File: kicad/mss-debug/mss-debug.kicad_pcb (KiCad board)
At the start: 2 copper layers, 82.6 x 76.2 mm, 94 parts, among them J1 Screw_Terminal_01x02, J10 Screw_Terminal_01x02, J2 SM04B-SRSS, J3 SM04B-SRSS, J4 SM04B-SRSS, J5 8P8C, J6 8P8C, J7 AVR-ISP, J8 Screw_Terminal_01x02, J9 Screw_Terminal_01x02, U1 AP7381-50Y, U2 ATtiny861A-S, U3 74HC4049, U4 AP3012

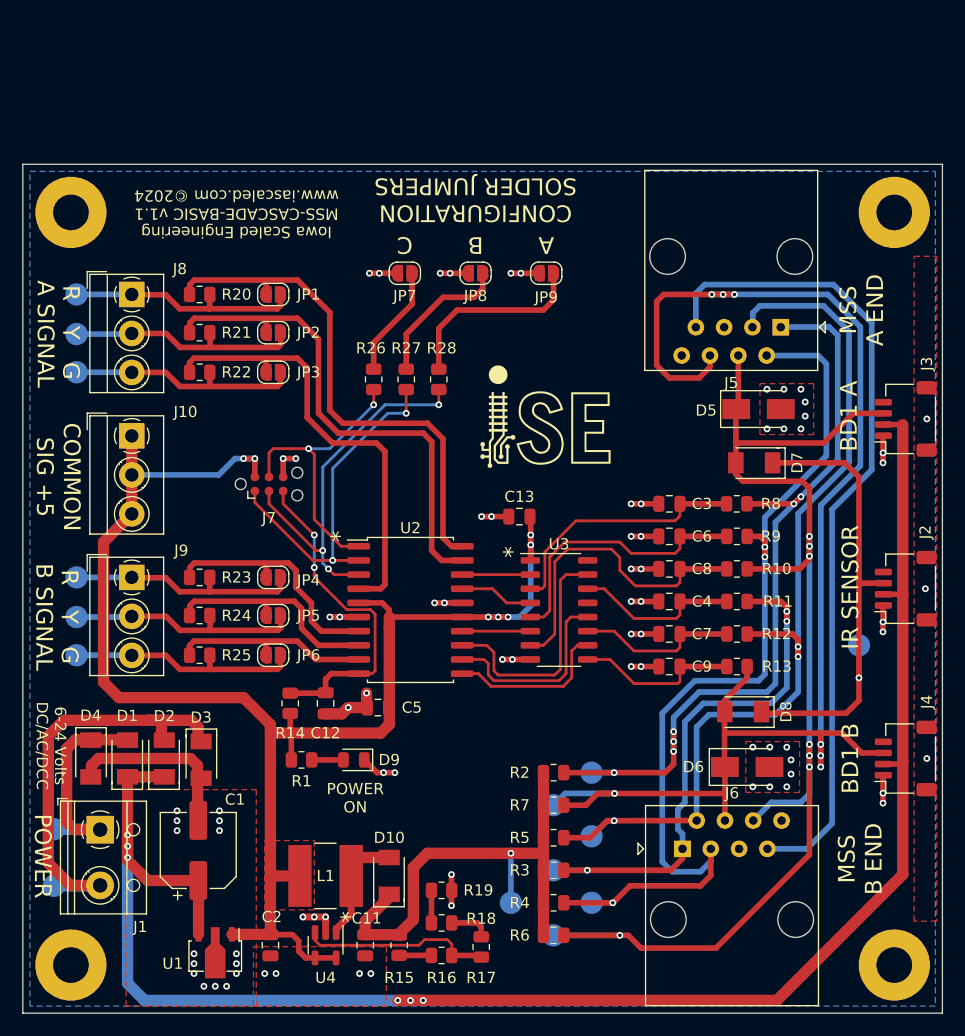
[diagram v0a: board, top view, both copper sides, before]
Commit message: Initial cut of the 2.0 board
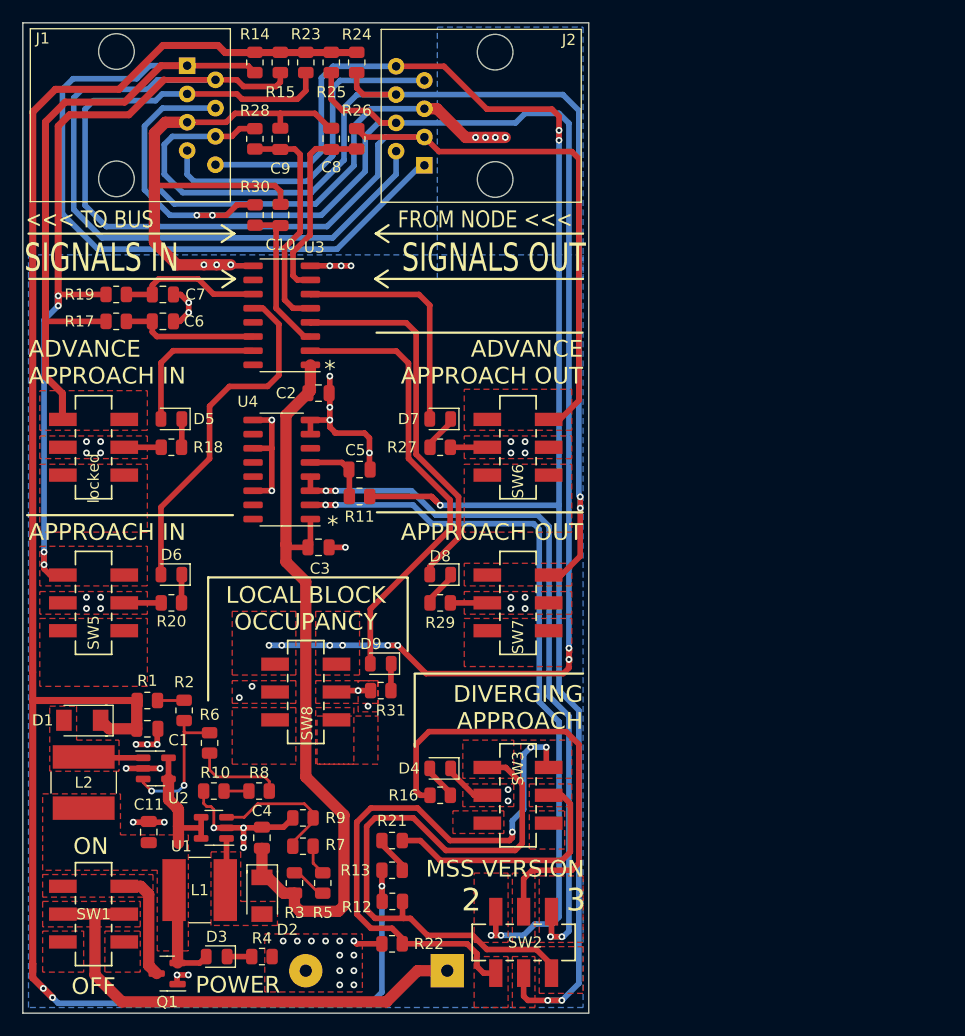
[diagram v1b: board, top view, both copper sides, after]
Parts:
- removed C12: 1uF, Capacitor_SMD:C_0805_2012Metric
- removed C13: 0.1uF, Capacitor_SMD:C_0805_2012Metric
- removed D10: CDBM140G, ISE_Generic:SOD-123T
- removed H1, H2, H3, H4: MountingHole, MountingHole:MountingHole_3.2mm_M3_Pad
- removed J10, J8, J9: Screw_Terminal_01x02, TerminalBlock_MetzConnect:TerminalBlock_MetzConnect_Type059_RT06303HBWC_1x03_P3.50mm_Horizontal
- removed J3, J4: SM04B-SRSS, Connector_JST:JST_SH_SM04B-SRSS-TB_1x04-1MP_P1.00mm_Horizontal
- removed J5, J6: 8P8C, Connector_RJ:RJ45_Amphenol_54602-x08_Horizontal
- removed J7: AVR-ISP, Connector:Tag-Connect_TC2030-IDC-NL_2x03_P1.27mm_Vertical
- removed JP1, JP2, JP3, JP4, JP5, JP6, JP7, JP8, JP9: SolderJumper_2_Open, Jumper:SolderJumper-2_P1.3mm_Open_RoundedPad1.0x1.5mm
- removed TP1, TP10, TP11, TP12, TP13, TP14, TP15, TP16, TP2, TP3, TP4, TP5, TP6, TP7, TP8, TP9: TestPoint, TestPoint:TestPoint_Pad_D2.0mm
- added BT1: Keystone 2479, Battery:BatteryHolder_Keystone_2479_3xAAA, B.Cu at (63.5, 188.0)
- added C10: 0.1uF, Capacitor_SMD:C_0805_2012Metric, F.Cu at (48.5, 120.1)
- added L2: 4.7uH, ISE_UltraLibrarian:MSS6132-xxxMLC, F.Cu at (30.9, 171.1)
- added Q1: Si2333, Package_TO_SOT_SMD:SOT-23, F.Cu at (38.4, 188.2)
- added R29: 1K, Resistor_SMD:R_0805_2012Metric, F.Cu at (62.9, 154.9)
- added R30: 10k, Resistor_SMD:R_0805_2012Metric, F.Cu at (46.2, 120.1)
- added R31: 1K, Resistor_SMD:R_0805_2012Metric, F.Cu at (57.5, 162.8)
- added SW1: JS202011SCQN, ISE_UltraLibrarian:SW_JS202011SCQN, F.Cu at (31.8, 182.9)
- added SW2: JS202011SCQN, ISE_UltraLibrarian:SW_JS202011SCQN, F.Cu at (70.4, 185.4)
- added SW3: JS202011SCQN, ISE_UltraLibrarian:SW_JS202011SCQN, F.Cu at (69.8, 172.2)
- added SW5: JS202011SCQN, ISE_UltraLibrarian:SW_JS202011SCQN, F.Cu at (31.8, 154.9)
- added SW6: JS202011SCQN, ISE_UltraLibrarian:SW_JS202011SCQN, F.Cu at (69.8, 141.0)
- added SW7: JS202011SCQN, ISE_UltraLibrarian:SW_JS202011SCQN, F.Cu at (69.8, 154.9)
- added SW8: JS202011SCQN, ISE_UltraLibrarian:SW_JS202011SCQN, F.Cu at (50.8, 162.9)
- added locked: JS202011SCQN, ISE_UltraLibrarian:SW_JS202011SCQN, F.Cu at (31.8, 141.0)
- C1: value 68uF -> 10uF; footprint Capacitor_SMD:CP_Elec_6.3x5.8 -> Capacitor_SMD:C_0805_2012Metric
- C11: value 10uF -> 22uF
- C2: value 22uF -> 0.1uF
- C4: value 0.1uF -> 10uF
- D3: value CDBM140G -> GREEN LED; footprint ISE_Generic:SOD-123T -> LED_SMD:LED_0805_2012Metric
- D4: value CDBM140G -> BLUE LED; footprint ISE_Generic:SOD-123T -> LED_SMD:LED_0805_2012Metric
- D5: value SMAJ18A-TP -> WHITE LED; footprint Diode_SMD:D_SMA -> LED_SMD:LED_0805_2012Metric
- D6: value SMAJ18A-TP -> YELLOW LED; footprint Diode_SMD:D_SMA -> LED_SMD:LED_0805_2012Metric
- D7: value CDBM140G -> WHITE LED; footprint ISE_Generic:SOD-123T -> LED_SMD:LED_0805_2012Metric
- D8: value CDBM140G -> YELLOW LED; footprint ISE_Generic:SOD-123T -> LED_SMD:LED_0805_2012Metric
- D9: value GREEN LED -> RED LED
- J1: value Screw_Terminal_01x02 -> 8P8C; footprint TerminalBlock_RND:TerminalBlock_RND_205-00012_1x02_P5.00mm_Horizontal -> Connector_RJ:RJ45_Amphenol_54602-x08_Horizontal
- J2: value SM04B-SRSS -> 8P8C; footprint Connector_JST:JST_SH_SM04B-SRSS-TB_1x04-1MP_P1.00mm_Horizontal -> Connector_RJ:RJ45_Amphenol_54602-x08_Horizontal
- R1, R17, R26, R28: value 1k -> 10k
- R10: value 10k -> 330
- R13, R16, R4, R6, R8: value 10k -> 1k
- R18, R27: value 1k -> 1K
- R19, R22, R23, R24, R25: value 330 -> 10k
- R20: value 330 -> 1K
- R21: value 330 -> 1k
- U1: value AP7381-50Y -> AP3012; footprint ISE_Generic:SOT-89-3 -> Package_TO_SOT_SMD:SOT-23-5
- U2: value ATtiny861A-S -> AP3012; footprint Package_SO:SOIC-20W_7.5x12.8mm_P1.27mm -> Package_TO_SOT_SMD:SOT-23-5
- U4: value AP3012 -> 74HC4049; footprint Package_TO_SOT_SMD:SOT-23-5 -> Package_SO:SO-16_3.9x9.9mm_P1.27mm
- moved R15 80.0 mm to (48.5, 106.4)
- moved J1 69.0 mm to (40.2, 106.7)
- moved R17 65.0 mm to (33.8, 129.7), turned to 180 degrees
- moved R19 60.9 mm to (33.8, 127.3)
- moved C9 58.9 mm to (48.5, 113.3), turned to 90 degrees
- moved R14 57.6 mm to (46.2, 106.4), turned to 90 degrees
- moved J2 57.5 mm to (61.4, 115.7)
- moved C7 54.7 mm to (38.0, 127.3), turned to 0 degrees
- moved R25 54.5 mm to (53.1, 106.4), turned to 90 degrees
- moved D6 54.5 mm to (38.7, 152.4), turned to 180 degrees
- moved R22 54.1 mm to (58.5, 185.5)
- moved D5 52.7 mm to (38.7, 138.4), turned to 180 degrees
- moved R24 51.6 mm to (55.4, 106.4), turned to 90 degrees
- moved R10 51.0 mm to (42.5, 171.8)
- moved R8 50.0 mm to (46.6, 171.8)
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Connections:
- C1 pad 1: /VPWR -> +12V
- C11 pad 1: +12V -> Net-(U1-Pad4)
- C3 pad 1: Net-(C3-Pad1) -> +5V
- C4 pad 1: Net-(C4-Pad1) -> +5V
- C5 pad 1: +5V -> Net-(C5-Pad1)
- D1 pad 1: /VPWR -> +12V
- D1 pad 2: Net-(D1-Pad2) -> Net-(L2-Pad2)
- D2 pad 1: /VPWR -> +5V
- D2 pad 2: Net-(D2-Pad2) -> Net-(U1-Pad1)
- D3 pad 1: Net-(D2-Pad2) -> Net-(D3-Pad1)
- D3 pad 2: GND -> Net-(U1-Pad4)
- D4 pad 1: Net-(D1-Pad2) -> GND
- D4 pad 2: GND -> Net-(D4-Pad2)
- D5 pad 1: /A_ADJACENT -> Net-(R18-Pad1)
- D5 pad 2: GND -> Net-(D5-Pad2)
- D6 pad 1: /B_ADJACENT -> Net-(R20-Pad1)
- D6 pad 2: GND -> Net-(D6-Pad2)
- D7 pad 1: Net-(D7-Pad1) -> Net-(R27-Pad1)
- D7 pad 2: /A_ADJACENT -> Net-(D7-Pad2)
- D8 pad 1: Net-(D7-Pad1) -> Net-(R29-Pad1)
- D8 pad 2: /B_ADJACENT -> Net-(D8-Pad2)
- D9 pad 1: GND -> Net-(D9-Pad1)
- J1 pad 1: Net-(D1-Pad2) -> /~{AA_IN}
- J1 pad 2: Net-(D2-Pad2) -> /~{A_IN}
- J2 pad 1: GND -> /~{AA_IN}
- J2 pad 2: /VPWR -> /~{A_IN}
- J2 pad 3: Net-(D7-Pad1) -> /~{AA_OUT}
- J2 pad 4: unconnected-(J2-Pad4) -> /~{LOCAL}
- L1 pad 1: +5V -> Net-(U1-Pad4)
- L1 pad 2: Net-(D10-Pad2) -> Net-(U1-Pad1)
- R1 pad 1: Net-(D9-Pad2) -> Net-(R1-Pad1)
- R1 pad 2: +5V -> +12V
- R10 pad 1: Net-(C8-Pad1) -> GND
- R10 pad 2: /A_ADJACENT -> Net-(R10-Pad2)
- R11 pad 1: Net-(C4-Pad1) -> Net-(C5-Pad1)
- R11 pad 2: Net-(J6-Pad1) -> /DVRG_APP
- R12 pad 1: Net-(C7-Pad1) -> Net-(R12-Pad1)
- R12 pad 2: Net-(J5-Pad3) -> +12V
- R13 pad 1: Net-(C9-Pad1) -> Net-(R13-Pad1)
- R13 pad 2: /B_ADJACENT -> +12V
- R14 pad 1: Net-(C12-Pad1) -> /~{AA_IN}
- R14 pad 2: +5V -> +12V
- R15 pad 1: Net-(R15-Pad1) -> /~{A_IN}
- R16 pad 1: Net-(R16-Pad1) -> Net-(D4-Pad2)
- R16 pad 2: Net-(R15-Pad1) -> Net-(R16-Pad2)
- R17 pad 1: Net-(R17-Pad1) -> Net-(C6-Pad1)
- R17 pad 2: Net-(R16-Pad1) -> /~{AA_IN}
- R18 pad 2: Net-(R17-Pad1) -> GND
- R19 pad 1: GND -> Net-(C7-Pad1)
- R19 pad 2: Net-(R18-Pad1) -> /~{A_IN}
- R2 pad 1: Net-(J5-Pad1) -> Net-(U2-Pad3)
- R2 pad 2: +12V -> Net-(R1-Pad1)
- R20 pad 1: /A_SIGNAL_R -> Net-(R20-Pad1)
- R20 pad 2: Net-(J8-Pad1) -> GND
- R21 pad 1: /A_SIGNAL_Y -> Net-(R21-Pad1)
- R21 pad 2: Net-(J8-Pad2) -> Net-(R13-Pad1)
- R22 pad 1: /A_SIGNAL_G -> GND
- R23 pad 1: /B_SIGNAL_R -> /~{AA_OUT}
- R23 pad 2: Net-(J9-Pad1) -> +12V
- R24 pad 1: /B_SIGNAL_Y -> /~{A_OUT}
- R24 pad 2: Net-(J9-Pad2) -> +12V
- R25 pad 1: /B_SIGNAL_G -> /~{LOCAL}
- R25 pad 2: Net-(J9-Pad3) -> +12V
- R26 pad 1: Net-(J7-Pad4) -> Net-(C8-Pad1)
- R26 pad 2: Net-(JP7-Pad1) -> /~{AA_OUT}
- R27 pad 1: Net-(J7-Pad1) -> Net-(R27-Pad1)
- R27 pad 2: Net-(JP8-Pad1) -> GND
- R28 pad 1: Net-(J7-Pad3) -> Net-(C9-Pad1)
- R28 pad 2: Net-(JP9-Pad1) -> /~{A_OUT}
- R3 pad 1: Net-(J6-Pad1) -> Net-(R3-Pad1)
- R3 pad 2: +12V -> +5V
- R4 pad 1: Net-(J5-Pad2) -> GND
- R4 pad 2: +12V -> Net-(D3-Pad1)
- R5 pad 1: Net-(J5-Pad3) -> Net-(R5-Pad1)
- R5 pad 2: +12V -> Net-(R3-Pad1)
- R6 pad 1: /A_ADJACENT -> Net-(R6-Pad1)
- R6 pad 2: +12V -> Net-(U2-Pad3)
- R7 pad 1: /B_ADJACENT -> Net-(U1-Pad3)
- R7 pad 2: +12V -> Net-(R5-Pad1)
- R8 pad 1: Net-(C3-Pad1) -> Net-(R10-Pad2)
- R8 pad 2: Net-(J5-Pad1) -> Net-(R6-Pad1)
- R9 pad 1: Net-(C6-Pad1) -> GND
- R9 pad 2: Net-(J5-Pad2) -> Net-(U1-Pad3)
- U1 pad 1: +5V -> Net-(U1-Pad1)
- U1 pad 3: /VPWR -> Net-(U1-Pad3)
- U2 pad 1: Net-(J7-Pad4) -> Net-(L2-Pad2)
- U2 pad 2: Net-(J7-Pad1) -> GND
- U2 pad 3: Net-(J7-Pad3) -> Net-(U2-Pad3)
- U2 pad 4: /A_SIGNAL_G -> Net-(U1-Pad4)
- U2 pad 5: +5V -> Net-(U1-Pad4)
- U3 pad 10: /B_ADJACENT_5V -> unconnected-(U3-Pad10)
- U3 pad 12: /B_APPROACH_5V -> Net-(D6-Pad2)
- U3 pad 14: Net-(C4-Pad1) -> Net-(C6-Pad1)
- U3 pad 15: /B_ADV_APPROACH_5V -> Net-(D5-Pad2)
- U3 pad 2: /A_ADV_APPROACH_5V -> Net-(D9-Pad2)
- U3 pad 3: Net-(C3-Pad1) -> Net-(C10-Pad1)
- U3 pad 4: /A_APPROACH_5V -> Net-(D8-Pad2)
- U3 pad 5: Net-(C6-Pad1) -> Net-(C9-Pad1)
- U3 pad 6: /A_ADJACENT_5V -> Net-(D7-Pad2)
- U3 pad 9: Net-(C9-Pad1) -> GND
- U4 pad 1: Net-(D10-Pad2) -> +5V
- U4 pad 2: GND -> Net-(SW2-Pad3)
- U4 pad 3: Net-(R16-Pad1) -> Net-(SW2-Pad1)
- U4 pad 4: +5V -> Net-(SW2-Pad1)
- U4 pad 5: +5V -> Net-(C5-Pad1)
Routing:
- net /VPWR: track 158.5 -> 0.00 mm, vias 6 -> 0
- net /~{LOCAL}: track 0.00 -> 151.5 mm, vias 0 -> 10
- net +12V: track 60.2 -> 211.2 mm, vias 1 -> 3
- net /DVRG_APP: track 0.00 -> 146.6 mm, vias 0 -> 5
- net /~{A_IN}: track 0.00 -> 129.4 mm, vias 0 -> 4
- net /B_ADJACENT: track 128.6 -> 0.00 mm, vias 7 -> 0
- net /A_ADJACENT: track 115.6 -> 0.00 mm, vias 7 -> 0
- net /~{AA_OUT}: track 0.00 -> 114.4 mm
- net /~{AA_IN}: track 0.00 -> 114.1 mm
- net GND: track 74.4 -> 181.0 mm, vias 81 -> 66
- net /~{A_OUT}: track 0.00 -> 106.0 mm, vias 0 -> 2
- net Net-(J5-Pad2): track 88.0 -> 0.00 mm, vias 3 -> 0
- net Net-(J5-Pad3): track 85.8 -> 0.00 mm, vias 3 -> 0
- net Net-(J5-Pad7): track 73.7 -> 0.00 mm
- net Net-(J5-Pad1): track 72.9 -> 0.00 mm, vias 6 -> 0
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- added copper zone on F.Cu, net /DVRG_APP
- added copper zone on F.Cu, net /~{AA_IN}
- added copper zone on F.Cu, net /~{AA_OUT}
- added copper zone on F.Cu, net /~{A_IN}
- added copper zone on F.Cu, net /~{A_OUT}
- added copper zone on F.Cu, net /~{LOCAL}
- added copper zone on F.Cu, net Net-(L2-Pad2)
- added copper zone on F.Cu, net Net-(R12-Pad1)
- added copper zone on F.Cu, net Net-(R16-Pad2)
- added copper zone on F.Cu, net Net-(R21-Pad1)
- added copper zone on F.Cu, net Net-(R22-Pad2)
- added copper zone on F.Cu, net Net-(SW1-Pad1)
- added copper zone on F.Cu, net Net-(SW1-Pad2)
- added copper zone on F.Cu, net Net-(SW2-Pad1)
- added copper zone on F.Cu, net Net-(SW2-Pad3)
- added copper zone on F.Cu, net Net-(SW4-Pad3)
- added copper zone on F.Cu, net Net-(SW5-Pad3)
- added copper zone on F.Cu, net Net-(SW6-Pad3)
- added copper zone on F.Cu, net Net-(SW7-Pad3)
- added copper zone on F.Cu, net Net-(U1-Pad1)
- added copper zone on F.Cu, net Net-(U1-Pad4)
- added copper zone on F.Cu, net unconnected-(SW1-Pad3)
- added copper zone on F.Cu, net unconnected-(SW1-Pad6)
- added copper zone on F.Cu, net unconnected-(SW3-Pad3)
- added copper zone on F.Cu, net unconnected-(SW3-Pad6)
- added copper zone on F.Cu, net unconnected-(SW8-Pad3)
- added copper zone on F.Cu, net unconnected-(SW8-Pad6)
- removed copper zone on F.Cu, net +5V
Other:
- board size 82.6 x 76.2 mm -> 50.8 x 88.9 mm
- board text added: "2"
- board text added: "3"
- board text added: "<<< TO BUS"
- board text added: "ADVANCE APPROACH IN"
- board text added: "ADVANCE APPROACH OUT"
- board text added: "APPROACH IN"
- board text added: "APPROACH OUT"
- board text added: "DIVERGING APPROACH"
- board text added: "FROM NODE <<<"
- board text added: "Iowa Scaled Engineering MSS-DEBUG v2.0 www.iascaled.com ©2024"
- board text added: "LOCAL BLOCK OCCUPANCY"
- board text added: "MSS VERSION"
- board text added: "OFF"
- board text added: "ON"
- board text added: "SIGNALS IN"
- board text added: "SIGNALS OUT"
- board text removed: "6-24 Volts DC/AC/DCC"
- board text removed: "A"
- board text removed: "A SIGNAL"
- board text removed: "B"
- board text removed: "B SIGNAL"
- board text removed: "BD1 A"
- board text removed: "BD1 B"
- board text removed: "C"
- board text removed: "COMMON SIG +5"
- board text removed: "CONFIGURATION SOLDER JUMPERS"
- board text removed: "G"
- board text removed: "IR SENSOR"
- board text removed: "Iowa Scaled Engineering MSS-CASCADE-BASIC v1.1 www.iascaled.com ©2024"
- board text removed: "MSS A END"
- board text removed: "MSS B END"
- board text removed: "POWER ON"
- board text removed: "R"
- board text removed: "Y"
